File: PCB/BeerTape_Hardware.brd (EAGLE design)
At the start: 63.5 x 80 mm, 6 parts

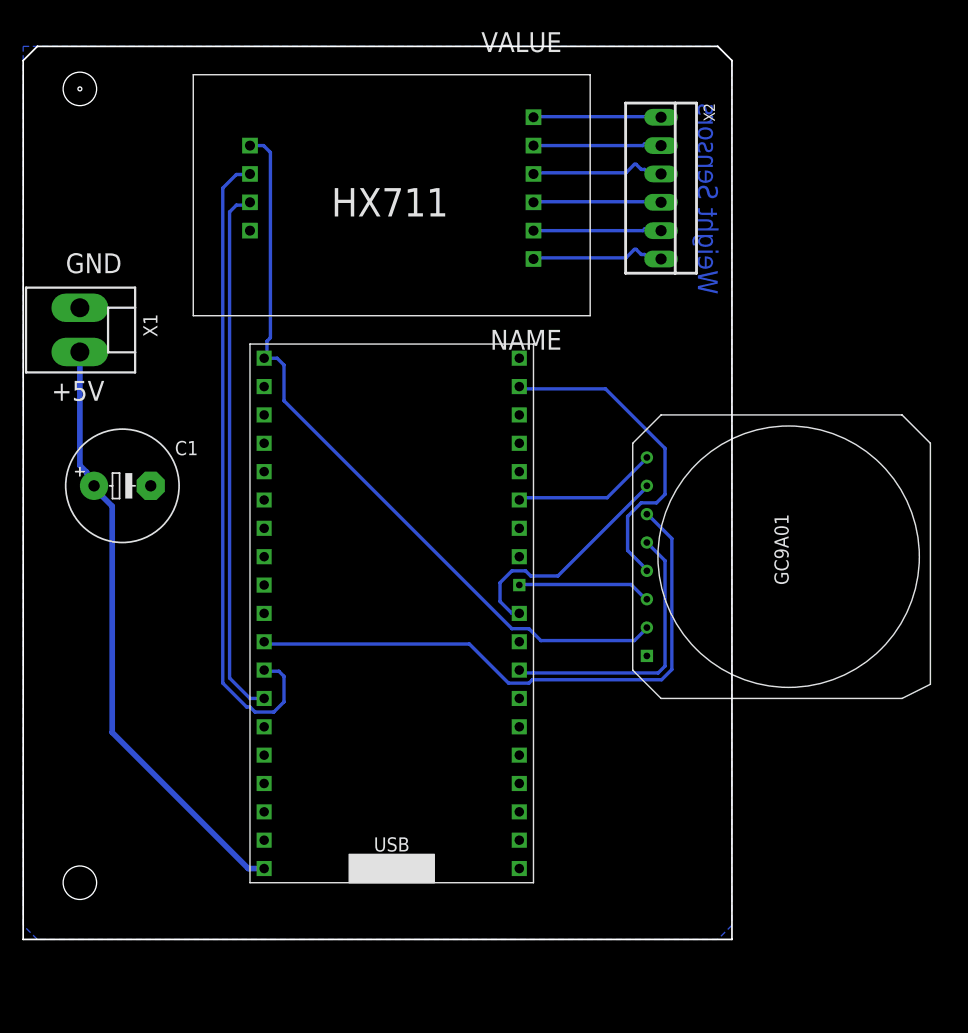
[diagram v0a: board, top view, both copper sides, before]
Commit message: PCB tested OK
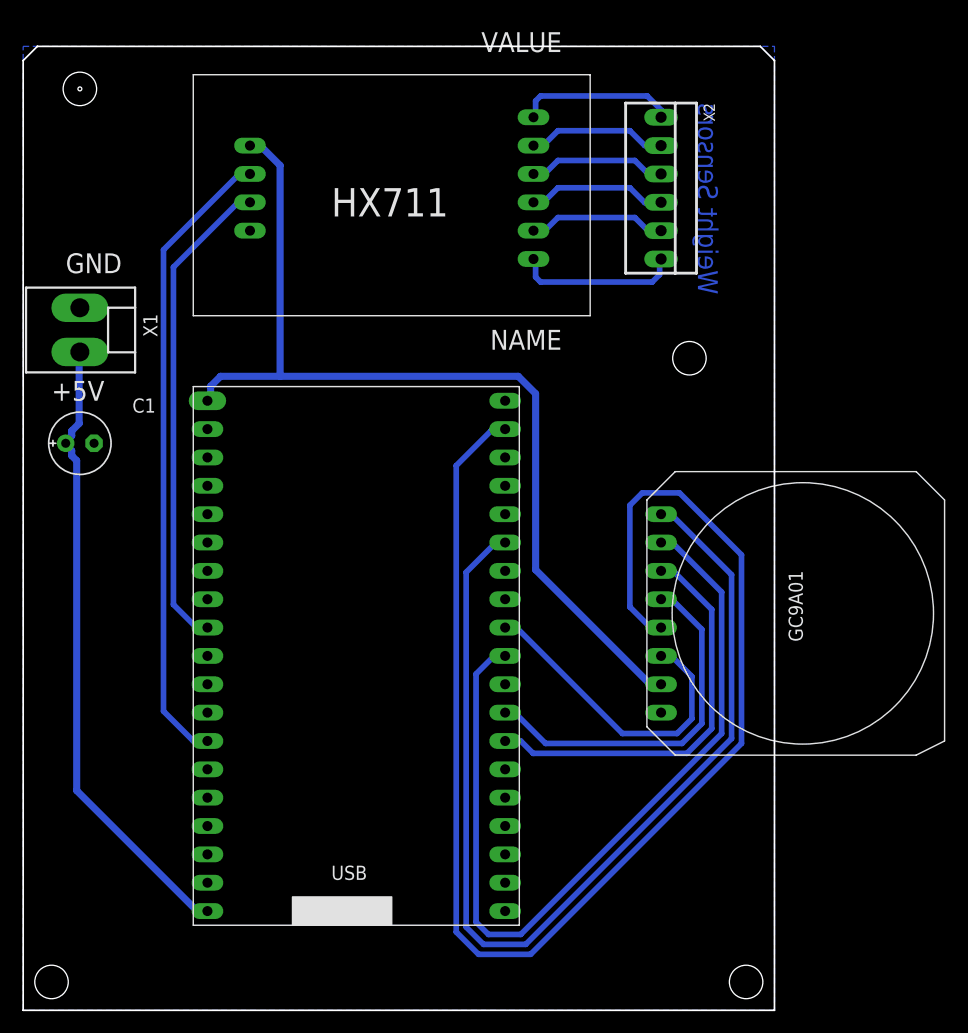
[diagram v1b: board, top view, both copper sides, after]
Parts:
- C1: device rcl:E5-10,5 -> rcl:E2,5-6E
- moved U$2 6.35 mm to (-8.89, -16.5)
- moved C1 5.39 mm to (-19.1, 26.7)
- moved U$1 5.24 mm to (33.0, 2.54)
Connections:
- removed net N$13: HX711.DT, U$2.GPIO12
- removed net N$14: HX711.SCK, U$2.GPIO14
- new net N$7: HX711.SCK, U$2.GPIO12
- new net N$8: HX711.DT, U$2.GPIO25
- net N$1: now also U$2.GPIO4; no longer U$2.GPIO27
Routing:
- net N$2: track 29.3 -> 124.0 mm
- net N$3: track 13.0 -> 91.7 mm
- net N$14: track 58.6 -> 0.00 mm
- net N$7: track 0.00 -> 56.9 mm
- net N$6: track 21.1 -> 75.3 mm
- net N$13: track 47.9 -> 0.00 mm
- net N$8: track 0.00 -> 43.4 mm
- net VCC: track 67.9 -> 85.1 mm
- net N$1: track 53.4 -> 36.5 mm
- net N$4: track 12.0 -> 28.6 mm
- net N$5: track 25.2 -> 32.7 mm
- net N$20: track 11.5 -> 14.2 mm
- net VDD: track 54.0 -> 56.8 mm
- net N$15: track 12.2 -> 14.8 mm
- net N$17: track 11.5 -> 12.5 mm
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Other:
- board size 63.5 x 80 mm -> 67.3 x 86.4 mm
